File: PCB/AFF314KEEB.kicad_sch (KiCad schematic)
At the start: 87 parts, among them SW1 RotaryEncoder_Switch, U1 Nice_Nano_V2

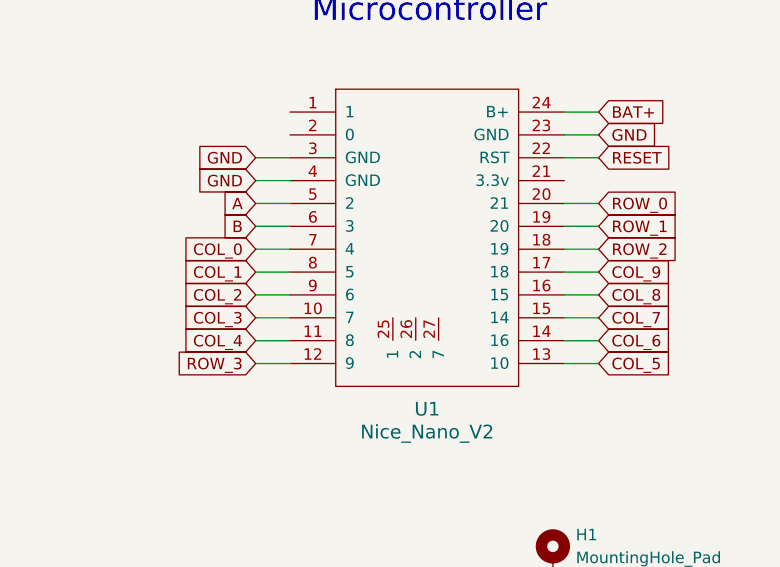
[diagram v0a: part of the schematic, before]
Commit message: Update
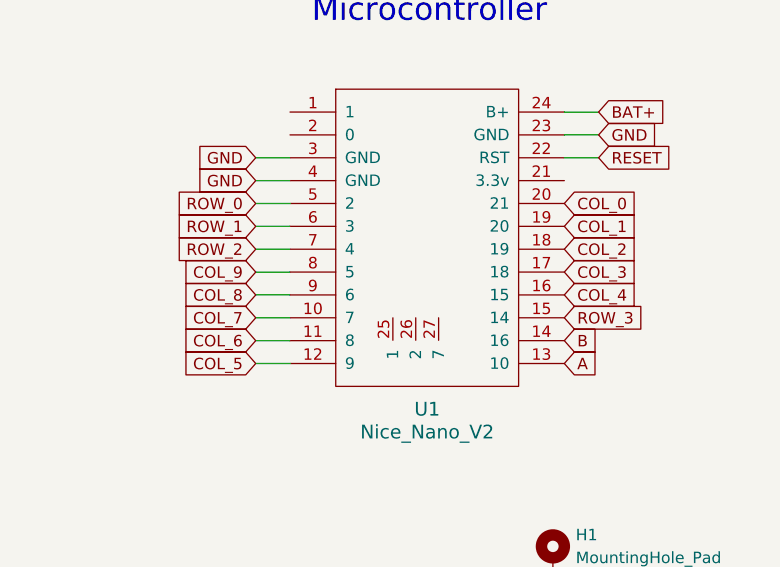
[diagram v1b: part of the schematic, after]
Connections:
- net A: now also U1.13 (10); no longer U1.5 (2)
- net B: now also U1.14 (16); no longer U1.6 (3)
- net COL_0: now also U1.20 (21); no longer U1.7 (4)
- net COL_1: now also U1.19 (20); no longer U1.8 (5)
- net COL_2: now also U1.18 (19); no longer U1.9 (6)
- net COL_3: now also U1.17 (18); no longer U1.10 (7)
- net COL_4: now also U1.16 (15); no longer U1.11 (8)
- net COL_5: now also U1.12 (9); no longer U1.13 (10)
- net COL_6: now also U1.11 (8); no longer U1.14 (16)
- net COL_7: now also U1.10 (7); no longer U1.15 (14)
- net COL_8: now also U1.9 (6); no longer U1.16 (15)
- net COL_9: now also U1.8 (5); no longer U1.17 (18)
- net ROW_0: now also U1.5 (2); no longer U1.20 (21)
- net ROW_1: now also U1.6 (3); no longer U1.19 (20)
- net ROW_2: now also U1.7 (4); no longer U1.18 (19)
- net ROW_3: now also U1.15 (14); no longer U1.12 (9)

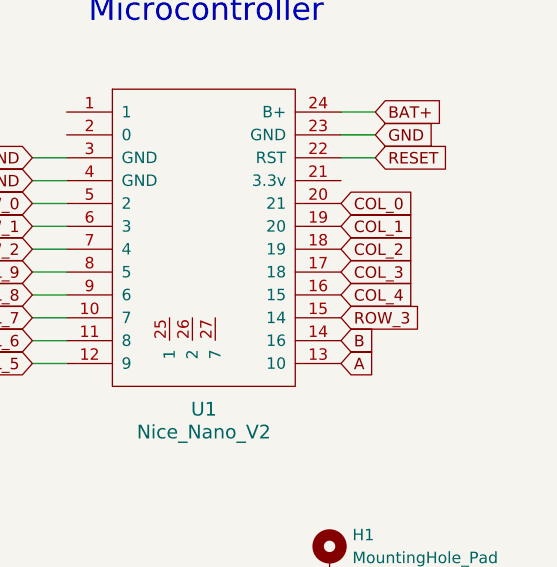
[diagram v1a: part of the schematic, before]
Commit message: Small PCB tweak
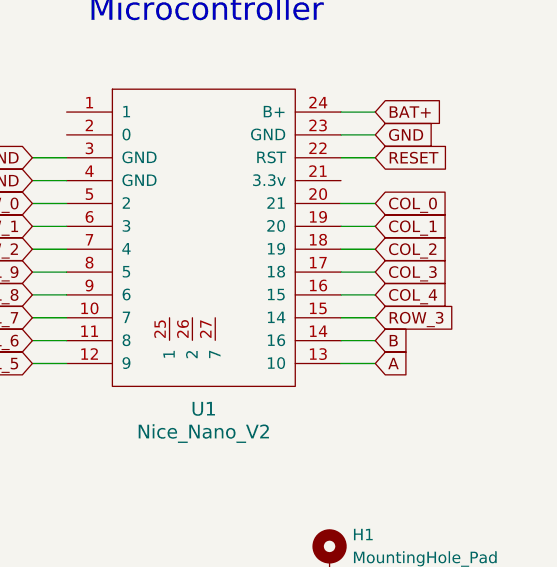
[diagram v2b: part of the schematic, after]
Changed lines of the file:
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@@
+	(wire
+		(pts
+			(xy 254 57.15) (xy 250.19 57.15)
+		)
+		(stroke
+			(width 0)
+			(type default)
+		)
+	)
 	(wire
 		(pts
@@
 	(wire
 		(pts
+			(xy 254 52.07) (xy 250.19 52.07)
+		)
+		(stroke
+			(width 0)
+			(type default)
+		)
+	)
+	(wire
+		(pts
 			(xy 93.98 90.17) (xy 93.98 107.95)
 		)
@@
 	(wire
 		(pts
+			(xy 254 54.61) (xy 250.19 54.61)
+		)
+		(stroke
+			(width 0)
+			(type default)
+		)
+	)
+	(wire
+		(pts
 			(xy 86.36 85.09) (xy 99.06 85.09)
 		)
@@
 	(wire
 		(pts
+			(xy 254 64.77) (xy 250.19 64.77)
+		)
+		(stroke
+			(width 0)
+			(type default)
+		)
+	)
+	(wire
+		(pts
 			(xy 119.38 46.99) (xy 119.38 54.61)
 		)
@@
 	(wire
 		(pts
+			(xy 254 59.69) (xy 250.19 59.69)
+		)
+		(stroke
+			(width 0)
+			(type default)
+		)
+	)
+	(wire
+		(pts
 			(xy 93.98 54.61) (xy 93.98 72.39)
 		)
@@
 	(wire
 		(pts
+			(xy 254 49.53) (xy 250.19 49.53)
+		)
+		(stroke
+			(width 0)
+			(type default)
+		)
+	)
+	(wire
+		(pts
+			(xy 254 62.23) (xy 250.19 62.23)
+		)
+		(stroke
+			(width 0)
+			(type default)
+		)
+	)
+	(wire
+		(pts
+			(xy 254 67.31) (xy 250.19 67.31)
+		)
+		(stroke
+			(width 0)
+			(type default)
+		)
+	)
+	(wire
+		(pts
 			(xy 137.16 67.31) (xy 149.86 67.31)
 		)
@@
 	(global_label "ROW_3"
 		(shape input)
-		(at 250.19 62.23 0)
-		(fields_autoplaced yes)
-		(effects
-			(font
-				(size 1.27 1.27)
-			)
-			(justify left)
-		)
-		(property "Intersheetrefs" "${INTERSHEET_REFS}"
-			(at 259.4042 62.23 0)
+		(at 254 62.23 0)
+		(fields_autoplaced yes)
+		(effects
+			(font
+				(size 1.27 1.27)
+			)
+			(justify left)
+		)
+		(property "Intersheetrefs" "${INTERSHEET_REFS}"
+			(at 263.2142 62.23 0)
 			(effects
 				(font
@@
 	(global_label "COL_4"
 		(shape input)
-		(at 250.19 59.69 0)
-		(fields_autoplaced yes)
-		(effects
-			(font
-				(size 1.27 1.27)
-			)
-			(justify left)
-		)
-		(property "Intersheetrefs" "${INTERSHEET_REFS}"
-			(at 258.9809 59.69 0)
+		(at 254 59.69 0)
+		(fields_autoplaced yes)
+		(effects
+			(font
+				(size 1.27 1.27)
+			)
+			(justify left)
+		)
+		(property "Intersheetrefs" "${INTERSHEET_REFS}"
+			(at 262.7909 59.69 0)
 			(effects
 				(font
@@
 	(global_label "A"
 		(shape input)
-		(at 250.19 67.31 0)
-		(fields_autoplaced yes)
-		(effects
-			(font
-				(size 1.27 1.27)
-			)
-			(justify left)
-		)
-		(property "Intersheetrefs" "${INTERSHEET_REFS}"
-			(at 254.2638 67.31 0)
+		(at 254 67.31 0)
+		(fields_autoplaced yes)
+		(effects
+			(font
+				(size 1.27 1.27)
+			)
+			(justify left)
+		)
+		(property "Intersheetrefs" "${INTERSHEET_REFS}"
+			(at 258.0738 67.31 0)
 			(effects
 				(font
@@
 	(global_label "B"
 		(shape input)
-		(at 250.19 64.77 0)
-		(fields_autoplaced yes)
-		(effects
-			(font
-				(size 1.27 1.27)
-			)
-			(justify left)
-		)
-		(property "Intersheetrefs" "${INTERSHEET_REFS}"
-			(at 254.4452 64.77 0)
+		(at 254 64.77 0)
+		(fields_autoplaced yes)
+		(effects
+			(font
+				(size 1.27 1.27)
+			)
+			(justify left)
+		)
+		(property "Intersheetrefs" "${INTERSHEET_REFS}"
+			(at 258.2552 64.77 0)
 			(effects
 				(font
@@
 	(global_label "COL_3"
 		(shape input)
-		(at 250.19 57.15 0)
-		(fields_autoplaced yes)
-		(effects
-			(font
-				(size 1.27 1.27)
-			)
-			(justify left)
-		)
-		(property "Intersheetrefs" "${INTERSHEET_REFS}"
-			(at 258.9809 57.15 0)
+		(at 254 57.15 0)
+		(fields_autoplaced yes)
+		(effects
+			(font
+				(size 1.27 1.27)
+			)
+			(justify left)
+		)
+		(property "Intersheetrefs" "${INTERSHEET_REFS}"
+			(at 262.7909 57.15 0)
 			(effects
 				(font
@@
 	(global_label "COL_0"
 		(shape input)
-		(at 250.19 49.53 0)
-		(fields_autoplaced yes)
-		(effects
-			(font
-				(size 1.27 1.27)
-			)
-			(justify left)
-		)
-		(property "Intersheetrefs" "${INTERSHEET_REFS}"
-			(at 258.9809 49.53 0)
+		(at 254 49.53 0)
+		(fields_autoplaced yes)
+		(effects
+			(font
+				(size 1.27 1.27)
+			)
+			(justify left)
+		)
+		(property "Intersheetrefs" "${INTERSHEET_REFS}"
+			(at 262.7909 49.53 0)
 			(effects
 				(font
@@
 	(global_label "COL_2"
 		(shape input)
-		(at 250.19 54.61 0)
-		(fields_autoplaced yes)
-		(effects
-			(font
-				(size 1.27 1.27)
-			)
-			(justify left)
-		)
-		(property "Intersheetrefs" "${INTERSHEET_REFS}"
-			(at 258.9809 54.61 0)
+		(at 254 54.61 0)
+		(fields_autoplaced yes)
+		(effects
+			(font
+				(size 1.27 1.27)
+			)
+			(justify left)
+		)
+		(property "Intersheetrefs" "${INTERSHEET_REFS}"
+			(at 262.7909 54.61 0)
 			(effects
 				(font
@@
 	(global_label "COL_1"
 		(shape input)
-		(at 250.19 52.07 0)
-		(fields_autoplaced yes)
-		(effects
-			(font
-				(size 1.27 1.27)
-			)
-			(justify left)
-		)
-		(property "Intersheetrefs" "${INTERSHEET_REFS}"
-			(at 258.9809 52.07 0)
-			(effects
-				(font
+		(at 254 52.07 0)
+		(fields_autoplaced yes)
+		(effects
+			(font
+				(size 1.27 1.27)
+			)
+			(justify left)
+		)
+		(property "Intersheetrefs" "${INTERSHEET_REFS}"
+			(at 262.7909 52.07 0)
+			(effects
+				(font
